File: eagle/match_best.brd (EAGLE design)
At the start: 10.2 x 59.2 mm, 7 parts, among them X1 SMA-142-0711-821/826

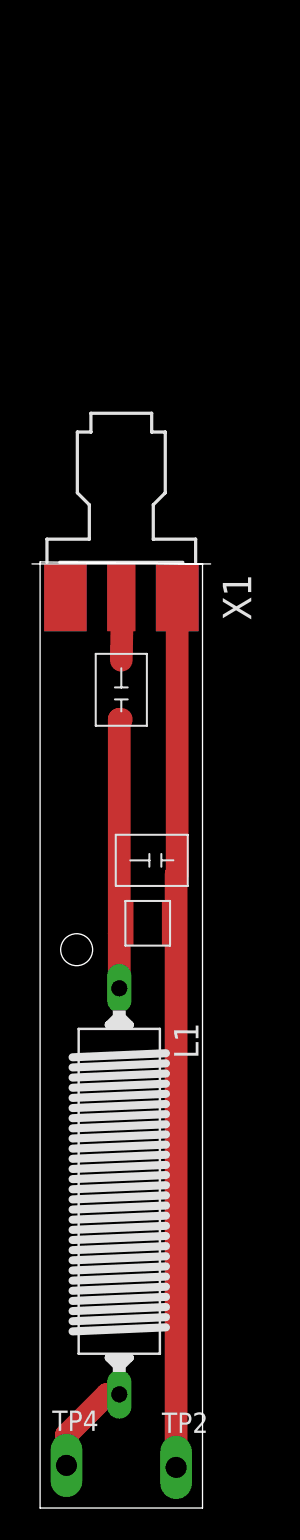
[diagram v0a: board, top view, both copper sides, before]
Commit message: asdfg
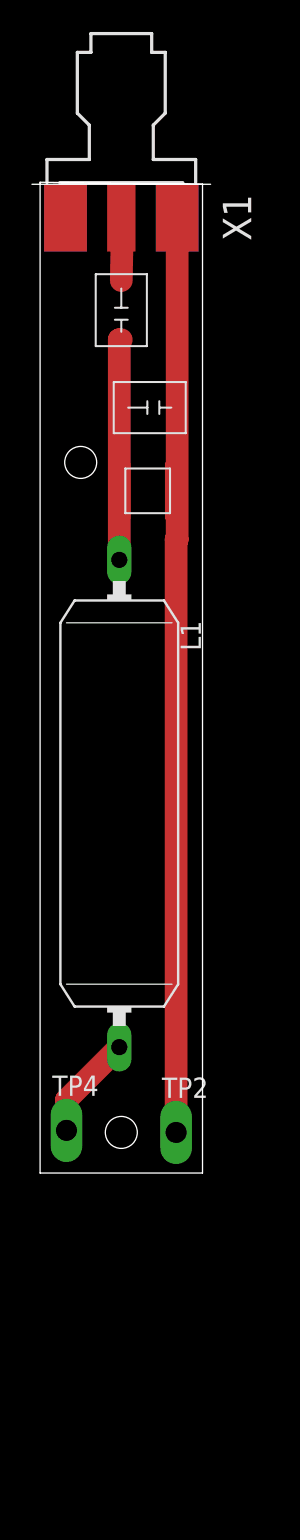
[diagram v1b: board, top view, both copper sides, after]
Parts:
- L1: value DRR1,5A -> B82111; device inductors:DR1,5A -> inductors:SUKW1-30
- moved C2 28.3 mm to (6.86, 47.9)
- moved C5 27.1 mm to (6.73, 42.7)
- moved L1 24.3 mm to (4.95, 23.1)
- moved C1 23.7 mm to (5.08, 54.0)
- moved X1 23.7 mm to (5.08, 61.8)
- moved TP2 21.0 mm to (8.51, 2.54)
- moved TP4 21.0 mm to (1.65, 2.67)
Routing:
- net N$1: track 16.9 -> 13.9 mm
- net N$2: track 54.5 -> 57.3 mm
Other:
- board size 10.2 x 59.2 mm -> 10.2 x 62 mm
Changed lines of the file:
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@@
 <board>
 <plain>
-<wire x1="0" y1="-20.955" x2="10.16" y2="-20.955" width="0" layer="20"/>
-<wire x1="10.16" y1="-20.955" x2="10.16" y2="38.1" width="0" layer="20"/>
-<wire x1="10.16" y1="38.1" x2="0" y2="38.227" width="0" layer="20"/>
-<wire x1="0" y1="38.227" x2="0" y2="-20.955" width="0" layer="20"/>
-<hole x="2.286" y="13.97" drill="2"/>
+<wire x1="0" y1="0" x2="10.16" y2="0" width="0" layer="20"/>
+<wire x1="10.16" y1="0" x2="10.16" y2="61.849" width="0" layer="20"/>
+<wire x1="10.16" y1="61.849" x2="0" y2="61.976" width="0" layer="20"/>
+<wire x1="0" y1="61.976" x2="0" y2="0" width="0" layer="20"/>
+<hole x="5.08" y="2.54" drill="2"/>
+<hole x="2.54" y="44.45" drill="2"/>
 </plain>
 <attributes>
@@
 </autorouter>
 <elements>
-<element name="C1" library="sprague" package="SGC3S" value="5-20" x="5.08" y="30.226" rot="R180"/>
-<element name="X1" library="con-coax" package="J502-ND-142-0711-821/826" value="SMA-142-0711-821/826" x="5.08" y="38.1" rot="R270">
-<attribute name="OC_NEWARK" value="16F3627" x="5.08" y="38.1" size="1.778" layer="27" rot="R270" display="off"/>
-<attribute name="MPN" value="142-0711-821" x="5.08" y="38.1" size="1.778" layer="27" rot="R270" display="off"/>
-<attribute name="MF" value="JOHNSON COMPONENTS" x="5.08" y="38.1" size="1.778" layer="27" rot="R270" display="off"/>
-<attribute name="OC_FARNELL" value="1019328" x="5.08" y="38.1" size="1.778" layer="27" rot="R270" display="off"/>
+<element name="C1" library="sprague" package="SGC3S" value="5-20" x="5.08" y="53.975" rot="R180"/>
+<element name="X1" library="con-coax" package="J502-ND-142-0711-821/826" value="SMA-142-0711-821/826" x="5.08" y="61.849" rot="R270">
+<attribute name="OC_NEWARK" value="16F3627" x="5.08" y="61.849" size="1.778" layer="27" rot="R270" display="off"/>
+<attribute name="MPN" value="142-0711-821" x="5.08" y="61.849" size="1.778" layer="27" rot="R270" display="off"/>
+<attribute name="MF" value="JOHNSON COMPONENTS" x="5.08" y="61.849" size="1.778" layer="27" rot="R270" display="off"/>
+<attribute name="OC_FARNELL" value="1019328" x="5.08" y="61.849" size="1.778" layer="27" rot="R270" display="off"/>
 </element>
-<element name="TP2" library="testpad" package="P1-13Y" value="TPPAD1-13Y" x="8.509" y="-18.415">
-<attribute name="TP_SIGNAL_NAME" value="" x="8.509" y="-18.415" size="1.778" layer="27" display="off"/>
+<element name="TP2" library="testpad" package="P1-13Y" value="TPPAD1-13Y" x="8.509" y="2.54">
+<attribute name="TP_SIGNAL_NAME" value="" x="8.509" y="2.54" size="1.778" layer="27" display="off"/>
 </element>
-<element name="TP4" library="testpad" package="P1-13Y" value="TPPAD1-13Y" x="1.651" y="-18.288">
-<attribute name="TP_SIGNAL_NAME" value="" x="1.651" y="-18.288" size="1.778" layer="27" display="off"/>
+<element name="TP4" library="testpad" package="P1-13Y" value="TPPAD1-13Y" x="1.651" y="2.667">
+<attribute name="TP_SIGNAL_NAME" value="" x="1.651" y="2.667" size="1.778" layer="27" display="off"/>
 </element>
-<element name="L1" library="inductors" package="DR1,5A" value="DRR1,5A" x="4.953" y="-1.143" rot="R270"/>
-<element name="C2" library="sprague" package="SGC3S" value="10-30" x="6.985" y="19.558" rot="R270"/>
-<element name="C5" library="resistor" package="1111" value="100p" x="6.731" y="15.621"/>
+<element name="L1" library="inductors" package="SUKW1-30" value="B82111" x="4.953" y="23.114" rot="R270"/>
+<element name="C2" library="sprague" package="SGC3S" value="10-30" x="6.858" y="47.879" rot="R270"/>
+<element name="C5" library="resistor" package="1111" value="100p" x="6.731" y="42.672"/>
 </elements>
 <signals>
@@
 <contactref element="C2" pad="P$2"/>
 <contactref element="C5" pad="P$1"/>
-<wire x1="5.08" y1="28.376" x2="4.953" y2="28.376" width="1.4224" layer="1"/>
-<wire x1="4.953" y1="28.376" x2="4.953" y2="14.986" width="1.4224" layer="1"/>
-<wire x1="4.953" y1="14.986" x2="4.953" y2="11.557" width="1.4224" layer="1"/>
-<wire x1="5.207" y1="15.621" x2="5.135" y2="19.558" width="0" layer="19" extent="1-1"/>
-<wire x1="4.953" y1="14.986" x2="5.207" y2="15.621" width="0" layer="19" extent="1-1"/>
+<wire x1="5.08" y1="52.125" x2="4.953" y2="52.125" width="1.4224" layer="1"/>
+<wire x1="4.953" y1="52.125" x2="4.953" y2="38.354" width="1.4224" layer="1"/>
+<wire x1="4.953" y1="35.941" x2="4.953" y2="38.354" width="0" layer="19" extent="1-16"/>
+<wire x1="4.953" y1="42.672" x2="5.008" y2="47.879" width="0" layer="19" extent="1-1"/>
+<wire x1="4.953" y1="35.941" x2="4.953" y2="42.672" width="0" layer="19" extent="1-1"/>
 </signal>
 <signal name="N$7">
 <contactref element="C1" pad="P$2"/>
 <contactref element="X1" pad="1"/>
-<wire x1="5.08" y1="35.9846" x2="5.152" y2="35.9846" width="1.4224" layer="1"/>
-<wire x1="5.152" y1="35.9846" x2="5.08" y2="32.076" width="1.4224" layer="1"/>
+<wire x1="5.08" y1="59.7336" x2="5.152" y2="59.7336" width="1.4224" layer="1"/>
+<wire x1="5.152" y1="59.7336" x2="5.08" y2="55.825" width="1.4224" layer="1"/>
 </signal>
 <signal name="N$2">
@@
 <contactref element="C2" pad="P$1"/>
 <contactref element="C5" pad="P$2"/>
-<wire x1="8.5746" y1="35.9846" x2="8.5746" y2="18.6754" width="1.4224" layer="1"/>
-<wire x1="8.5746" y1="18.6754" x2="8.509" y2="18.6754" width="1.4224" layer="1"/>
-<wire x1="8.509" y1="18.6754" x2="8.509" y2="-18.415" width="1.4224" layer="1"/>
-<wire x1="8.5746" y1="35.9846" x2="8.5746" y2="35.9846" width="0" layer="19" extent="1-16"/>
-<wire x1="8.835" y1="19.558" x2="8.5746" y2="18.6754" width="0" layer="19" extent="1-1"/>
-<wire x1="8.255" y1="15.621" x2="8.5746" y2="18.6754" width="0" layer="19" extent="1-1"/>
-<wire x1="1.5854" y1="35.9846" x2="8.5746" y2="35.9846" width="0" layer="19" extent="1-16"/>
-<wire x1="1.5854" y1="35.9846" x2="1.5854" y2="35.9846" width="0" layer="19" extent="1-16"/>
+<wire x1="8.5746" y1="59.7336" x2="8.5746" y2="39.6304" width="1.4224" layer="1"/>
+<wire x1="8.5746" y1="39.6304" x2="8.509" y2="39.6304" width="1.4224" layer="1"/>
+<wire x1="8.509" y1="39.6304" x2="8.509" y2="2.54" width="1.4224" layer="1"/>
+<wire x1="8.5746" y1="59.7336" x2="8.5746" y2="59.7336" width="0" layer="19" extent="1-16"/>
+<wire x1="8.708" y1="47.879" x2="8.5746" y2="39.6304" width="0" layer="19" extent="1-1"/>
+<wire x1="8.509" y1="42.672" x2="8.5746" y2="39.6304" width="0" layer="19" extent="1-1"/>
+<wire x1="1.5854" y1="59.7336" x2="8.5746" y2="59.7336" width="0" layer="19" extent="1-16"/>
+<wire x1="1.5854" y1="59.7336" x2="1.5854" y2="59.7336" width="0" layer="19" extent="1-16"/>
 </signal>
 <signal name="N$3">
 <contactref element="TP4" pad="TP"/>
 <contactref element="L1" pad="2"/>
-<wire x1="4.953" y1="-13.843" x2="4.191" y2="-13.843" width="1.4224" layer="1"/>
-<wire x1="4.191" y1="-13.843" x2="1.651" y2="-16.383" width="1.4224" layer="1"/>
-<wire x1="1.651" y1="-16.383" x2="1.651" y2="-18.288" width="1.4224" layer="1"/>
+<wire x1="4.953" y1="7.874" x2="1.651" y2="4.572" width="1.4224" layer="1"/>
+<wire x1="1.651" y1="4.572" x2="1.651" y2="2.667" width="1.4224" layer="1"/>
 </signal>
 </signals>
